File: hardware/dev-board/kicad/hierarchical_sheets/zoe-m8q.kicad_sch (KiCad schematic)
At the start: 38 parts, among them J1 CONSMA020.062-G, U5 ZOE-M8Q, Y1 32.768kHz

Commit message: file sync
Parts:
- JP?: footprint Jumper:SolderJumper-3_P1.3mm_Bridged12_RoundedPad1.0x1.5mm -> Jumper:SolderJumper-3_P1.3mm_Open_RoundedPad1.0x1.5mm
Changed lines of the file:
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@@
       (effects (font (size 1.27 1.27)) hide)
     )
-    (property "Footprint" "Jumper:SolderJumper-3_P1.3mm_Bridged12_RoundedPad1.0x1.5mm" (id 2) (at 201.93 156.845 0)
+    (property "Footprint" "Jumper:SolderJumper-3_P1.3mm_Open_RoundedPad1.0x1.5mm" (id 2) (at 201.93 156.845 0)
       (effects (font (size 1.27 1.27)) hide)
     )

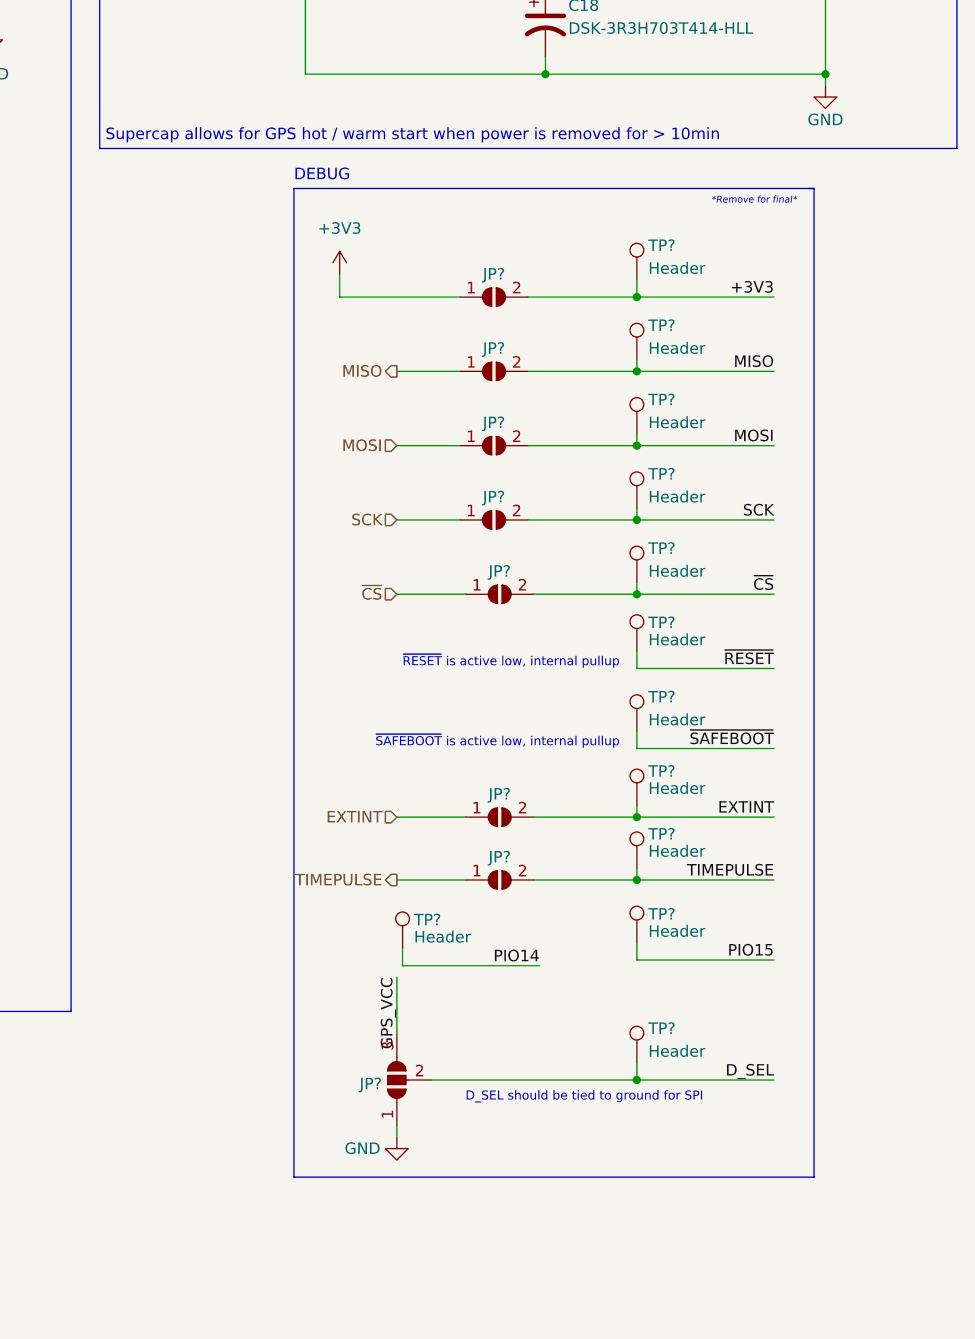
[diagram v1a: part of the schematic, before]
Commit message: rf is hard
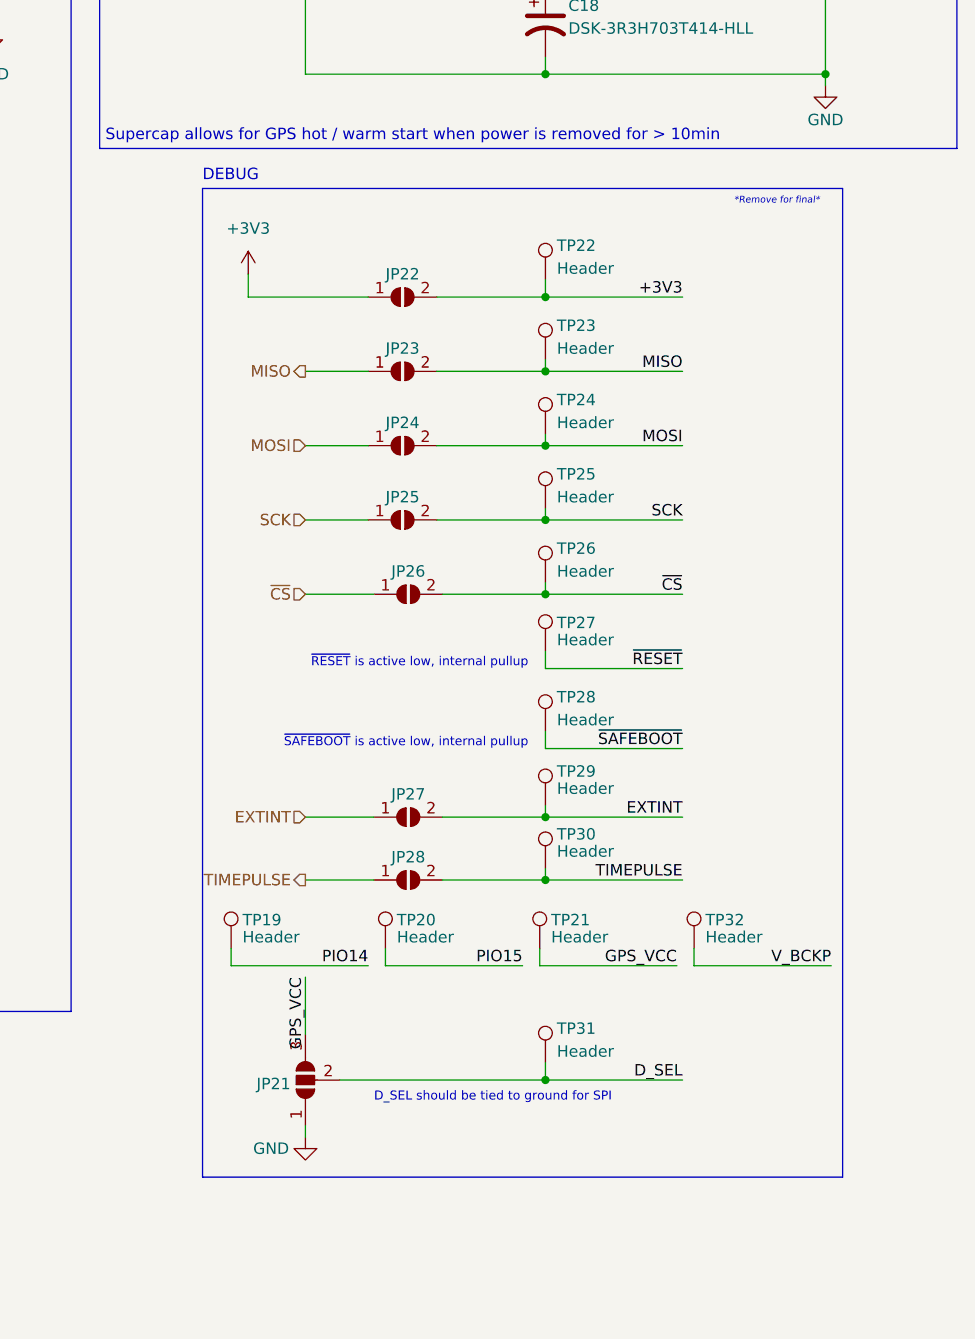
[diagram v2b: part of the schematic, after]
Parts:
- added TP21, TP32: Header, Connector_PinHeader_2.54mm:PinHeader_1x01_P2.54mm_Vertical, symbol Connector:TestPoint
- gave numbers to parts that had none: 20
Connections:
- net GPS_VCC: now also TP21.1
- net V_BCKP: now also TP32.1
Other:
- moved on the sheet: JP21, JP22, JP23, JP24, JP25, JP26, JP27, JP28, TP19, TP20, TP22, TP23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
